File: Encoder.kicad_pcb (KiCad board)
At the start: 2 copper layers, 23.2 x 26.5 mm, 17 parts, among them J1 Conn_01x05_Pin, SW1 RotaryEncoder_Switch_MP, U1 74LVC3G14

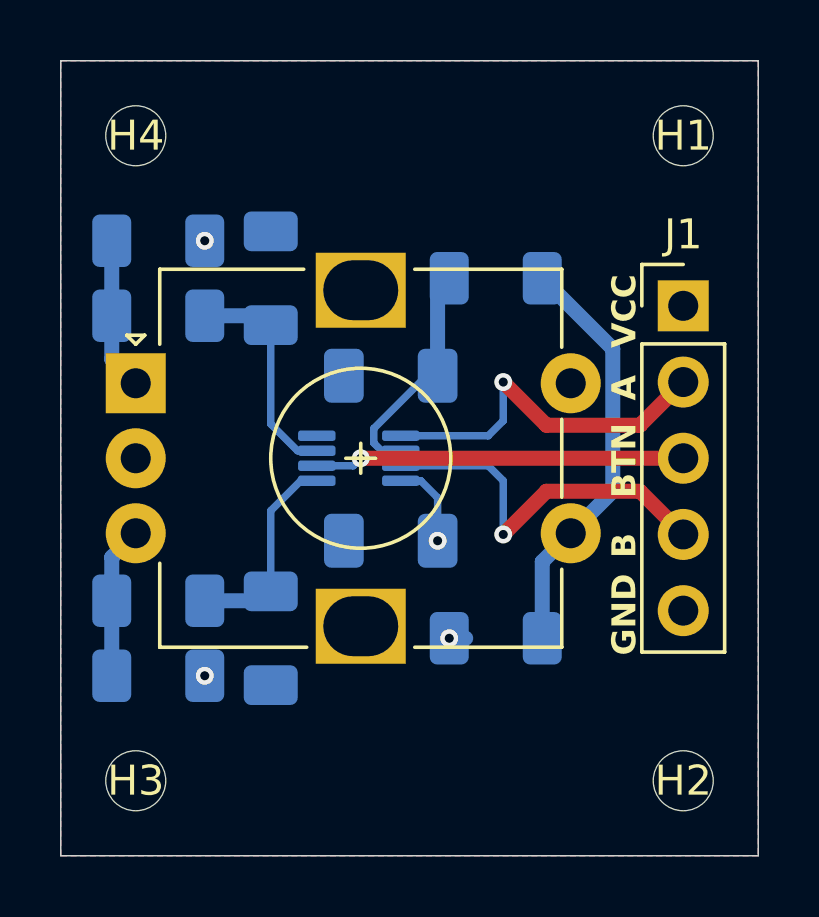
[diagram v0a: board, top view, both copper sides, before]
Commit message: Address warnings
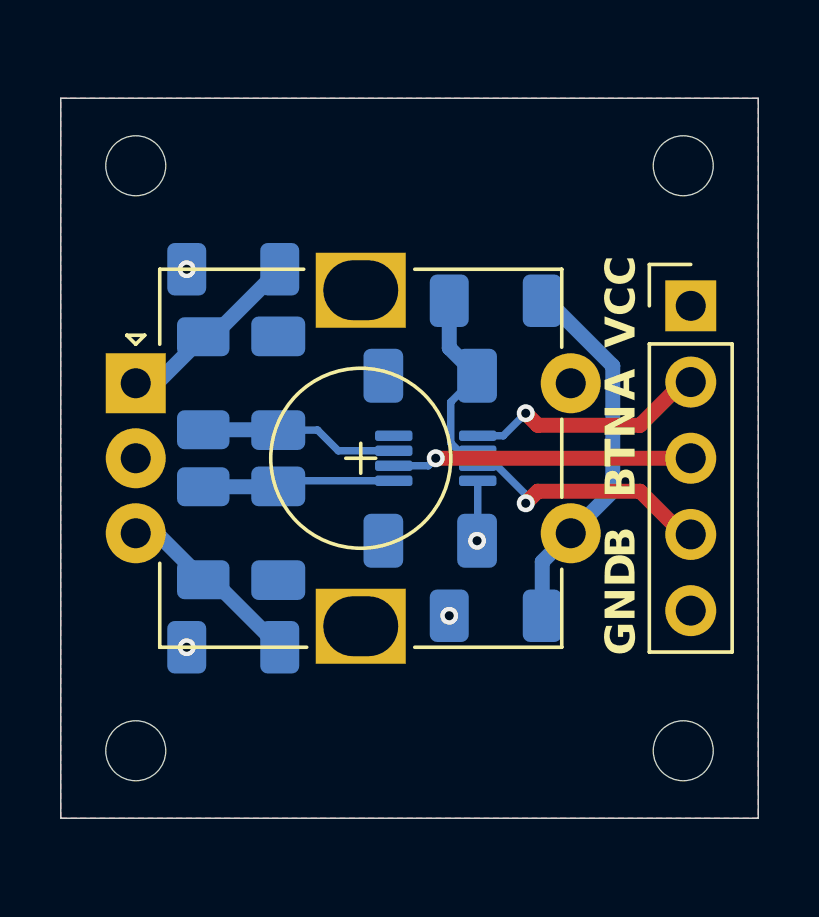
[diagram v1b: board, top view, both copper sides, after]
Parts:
- moved C2 3.51 mm to (149.8, 108.8)
- moved C3 3.51 mm to (149.8, 113.8)
- moved R3 2.70 mm to (147.2, 108.8), turned to -90 degrees
- moved R5 2.70 mm to (147.2, 113.8), turned to -90 degrees
- moved R4 2.67 mm to (148.2, 105.0), turned to 0 degrees
- moved R6 2.67 mm to (148.2, 117.5), turned to 0 degrees
- moved U1 2.56 mm to (155.0, 111.2)
- moved C1 1.31 mm to (154.8, 108.5)
- moved C4 1.31 mm to (154.8, 114.0)
- moved H1 1.00 mm to (163.2, 101.5)
- moved H2 1.00 mm to (163.2, 121.0)
- moved H3 1.00 mm to (145.0, 121.0)
- moved H4 1.00 mm to (145.0, 101.5)
- moved R1 0.75 mm to (157.0, 116.5)
- moved R2 0.75 mm to (157.0, 106.0)
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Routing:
- net /Debounced.B: track 12.6 -> 8.30 mm
- net /Debounced.A: track 12.1 -> 7.92 mm
- net /Debounced.BTN: track 12.3 -> 9.75 mm
- net VCC: track 3.45 -> 2.01 mm
- net /BTN: track 13.9 -> 12.6 mm
- net /B: track 5.08 -> 6.37 mm
- net /A: track 5.08 -> 6.37 mm
- net Net-(C1-Pad1): track 7.76 -> 6.50 mm
- net Net-(C2-Pad1): track 7.53 -> 6.64 mm
- net Net-(C3-Pad1): track 6.97 -> 6.43 mm
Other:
- board size 23.2 x 26.5 mm -> 23.2 x 24 mm
